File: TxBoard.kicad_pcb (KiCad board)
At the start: 2 copper layers, 94 x 31.7 mm, 22 parts, among them J1 RCA Socket, Q1 RU1J002YNTCL, SW1 Pull-Up, SW2 Input(Hi-Z)/Output, SW3 High/Low

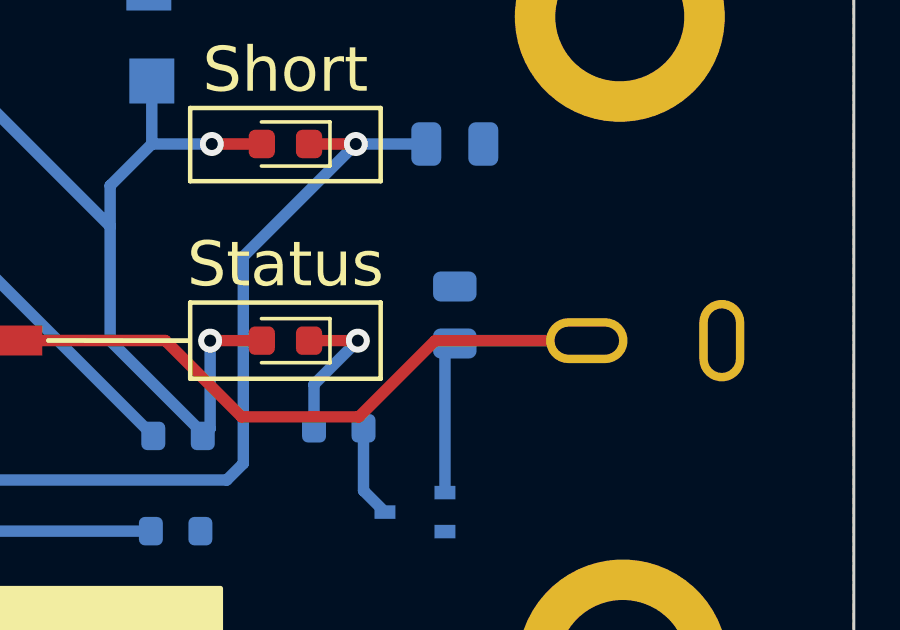
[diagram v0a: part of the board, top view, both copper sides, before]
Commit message: Production Run 0
Only a matter of time!
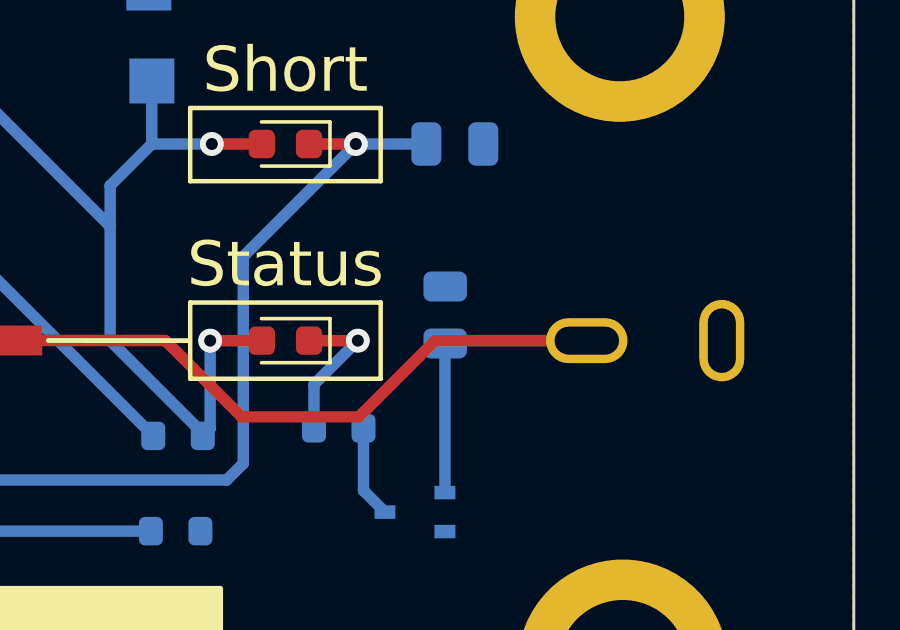
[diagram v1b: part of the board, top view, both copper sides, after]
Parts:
- moved C1 0.32 mm to (183.4, 96.3)
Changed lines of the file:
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@@
   )
   (footprint "Capacitor_SMD:C_0805_2012Metric" (layer "B.Cu")
-    (at 183.7 96.3 90)
+    (at 183.38 96.3 90)
     (descr "Capacitor SMD 0805 (2012 Metric), square (rectangular) end terminal, IPC_7351 nominal, (Body size source: IPC-SM-782 page 76, https://www.pcb-3d.com/wordpress/wp-content/uploads/ipc-sm-782a_amendment_1_and_2.pdf, https://docs.google.com/spreadsheets/d/1BsfQQcO9C6DZCsRaXUlFlo91Tg2WpOkGARC1WS5S8t0/edit?usp=sharing), generated with kicad-footprint-generator")
     (tags "capacitor")
@@
       (stroke (width 0.05) (type solid)) (layer "B.CrtYd"))
     (pad "1" smd rect (at 0 0 180) (size 1.5 1.5) (layers "B.Cu" "B.Mask")
-      (net 2 "GND") (pinfunction "1") (pintype "passive"))
+      (net 2 "GND") (pinfunction "1") (pintype "passive") (zone_connect 2))
   )
   (gr_rect (start 120.463 100.375) (end 121.733 102.915)
